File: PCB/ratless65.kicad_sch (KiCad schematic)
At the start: 134 parts, among them J1 MJ-4PP-9, J2 MJ-4PP-9, U1 ProMicro, U2 ProMicro

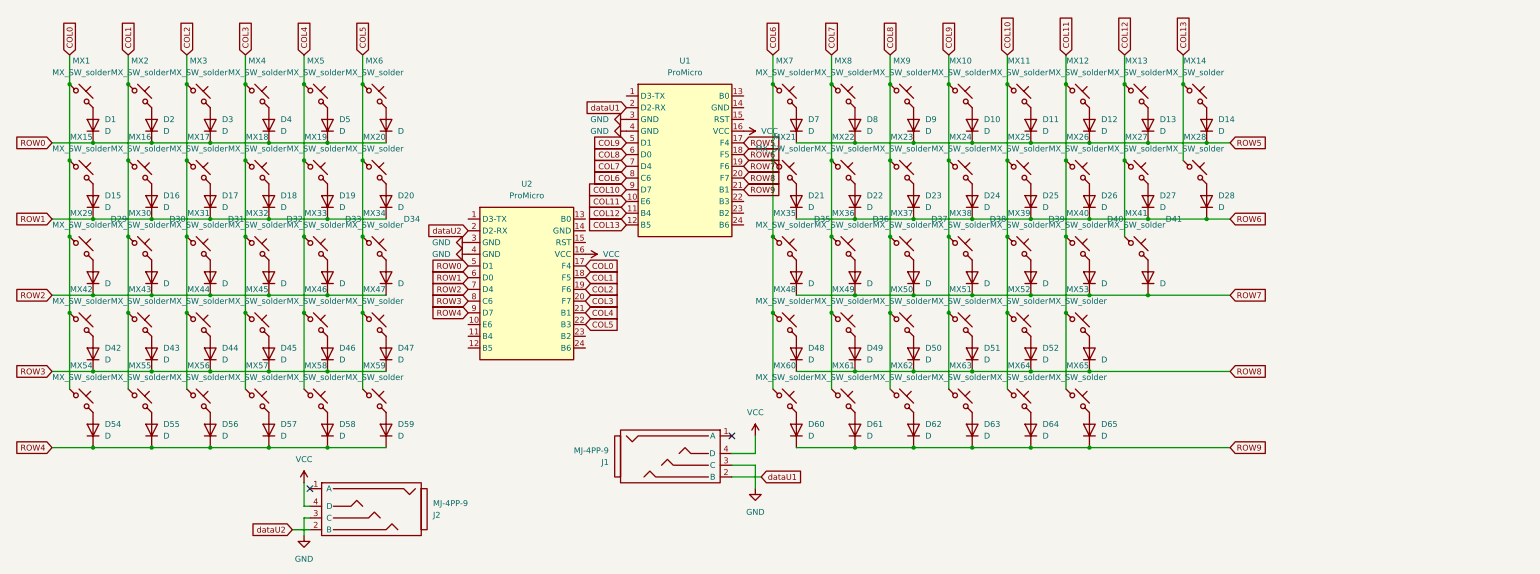
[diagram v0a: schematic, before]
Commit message: I have no clue what changed but just want everything synced
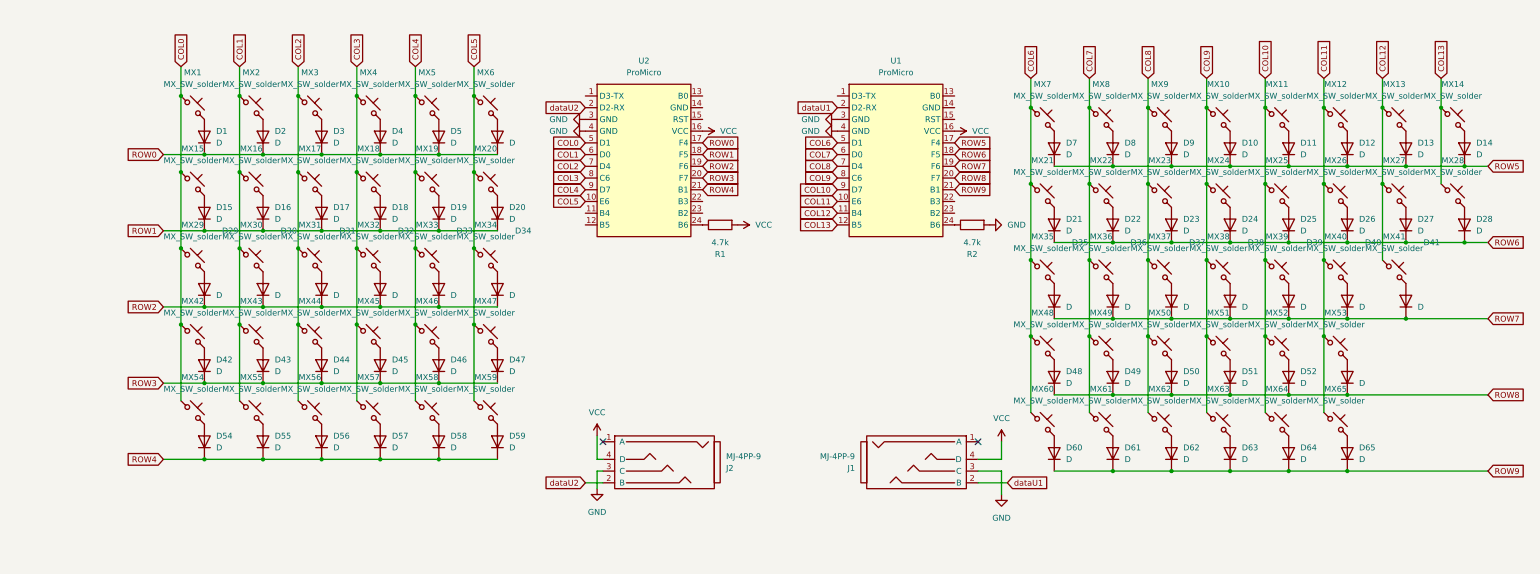
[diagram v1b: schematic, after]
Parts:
- added R1, R2: 4.7k, PCM_Resistor_SMD_AKL:R_1206_3216Metric, symbol Device:R
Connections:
- net COL0: now also U2.5 (D1); no longer U2.17 (F4)
- net COL1: now also U2.6 (D0); no longer U2.18 (F5)
- net COL2: now also U2.7 (D4); no longer U2.19 (F6)
- net COL3: now also U2.8 (C6); no longer U2.20 (F7)
- net COL4: now also U2.9 (D7); no longer U2.21 (B1)
- net COL5: now also U2.10 (E6); no longer U2.22 (B3)
- net COL6: now also U1.5 (D1); no longer U1.8 (C6)
- net COL7: now also U1.6 (D0); no longer U1.7 (D4)
- net COL8: now also U1.7 (D4); no longer U1.6 (D0)
- net COL9: now also U1.8 (C6); no longer U1.5 (D1)
- net GND: now also R2.2
- net ROW0: now also U2.17 (F4); no longer U2.5 (D1)
- net ROW1: now also U2.18 (F5); no longer U2.6 (D0)
- net ROW2: now also U2.19 (F6); no longer U2.7 (D4)
- net ROW3: now also U2.20 (F7); no longer U2.8 (C6)
- net ROW4: now also U2.21 (B1); no longer U2.9 (D7)
- net VCC: now also R1.2
- net at U1.24 (B6): now also R2.1
- net at U2.24 (B6): now also R1.1
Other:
- moved on the sheet: D1, D10, D11, D12, D13, D14, D15, D16, D17, D18, D19, D2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
